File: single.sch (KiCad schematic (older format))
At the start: 8 parts, among them J1 Conn_01x01, J2 Conn_01x01, J3 Conn_01x01, J4 Conn_01x01, J5 Conn_01x01, J6 Conn_01x01

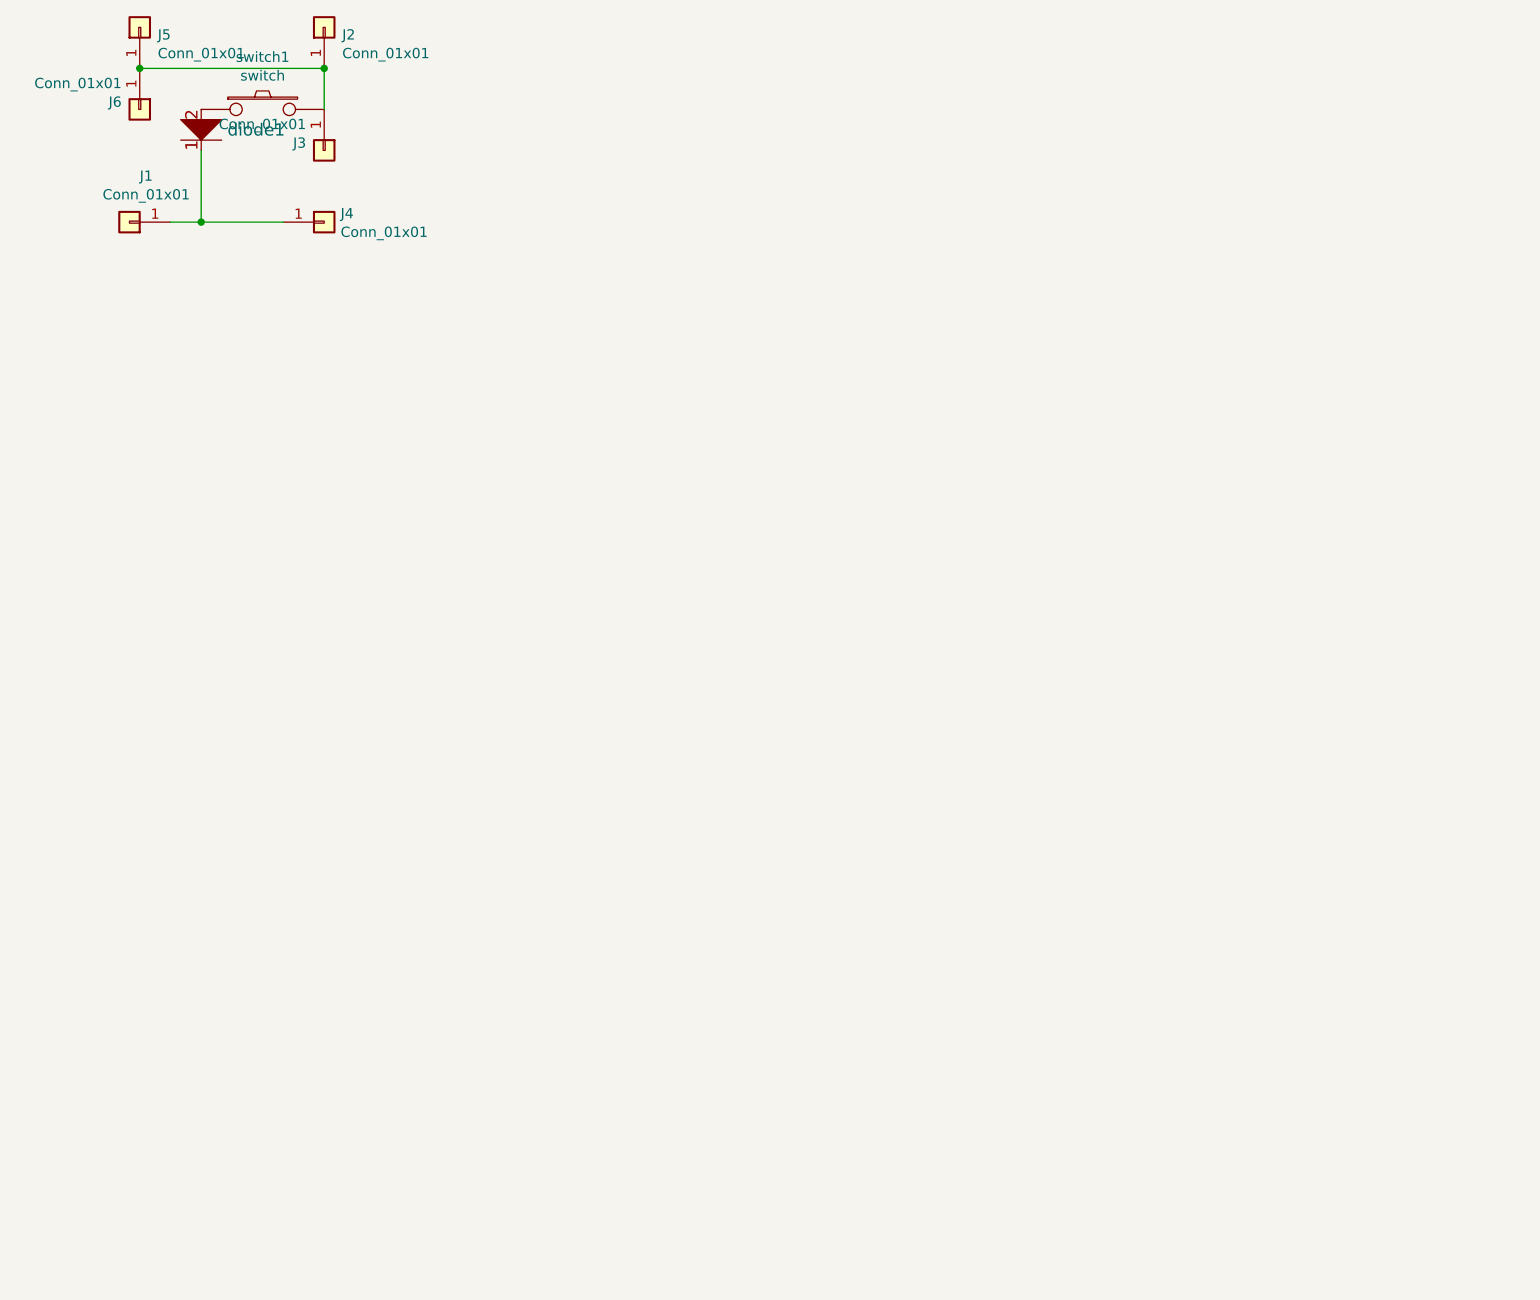
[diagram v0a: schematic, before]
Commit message: 6x5.
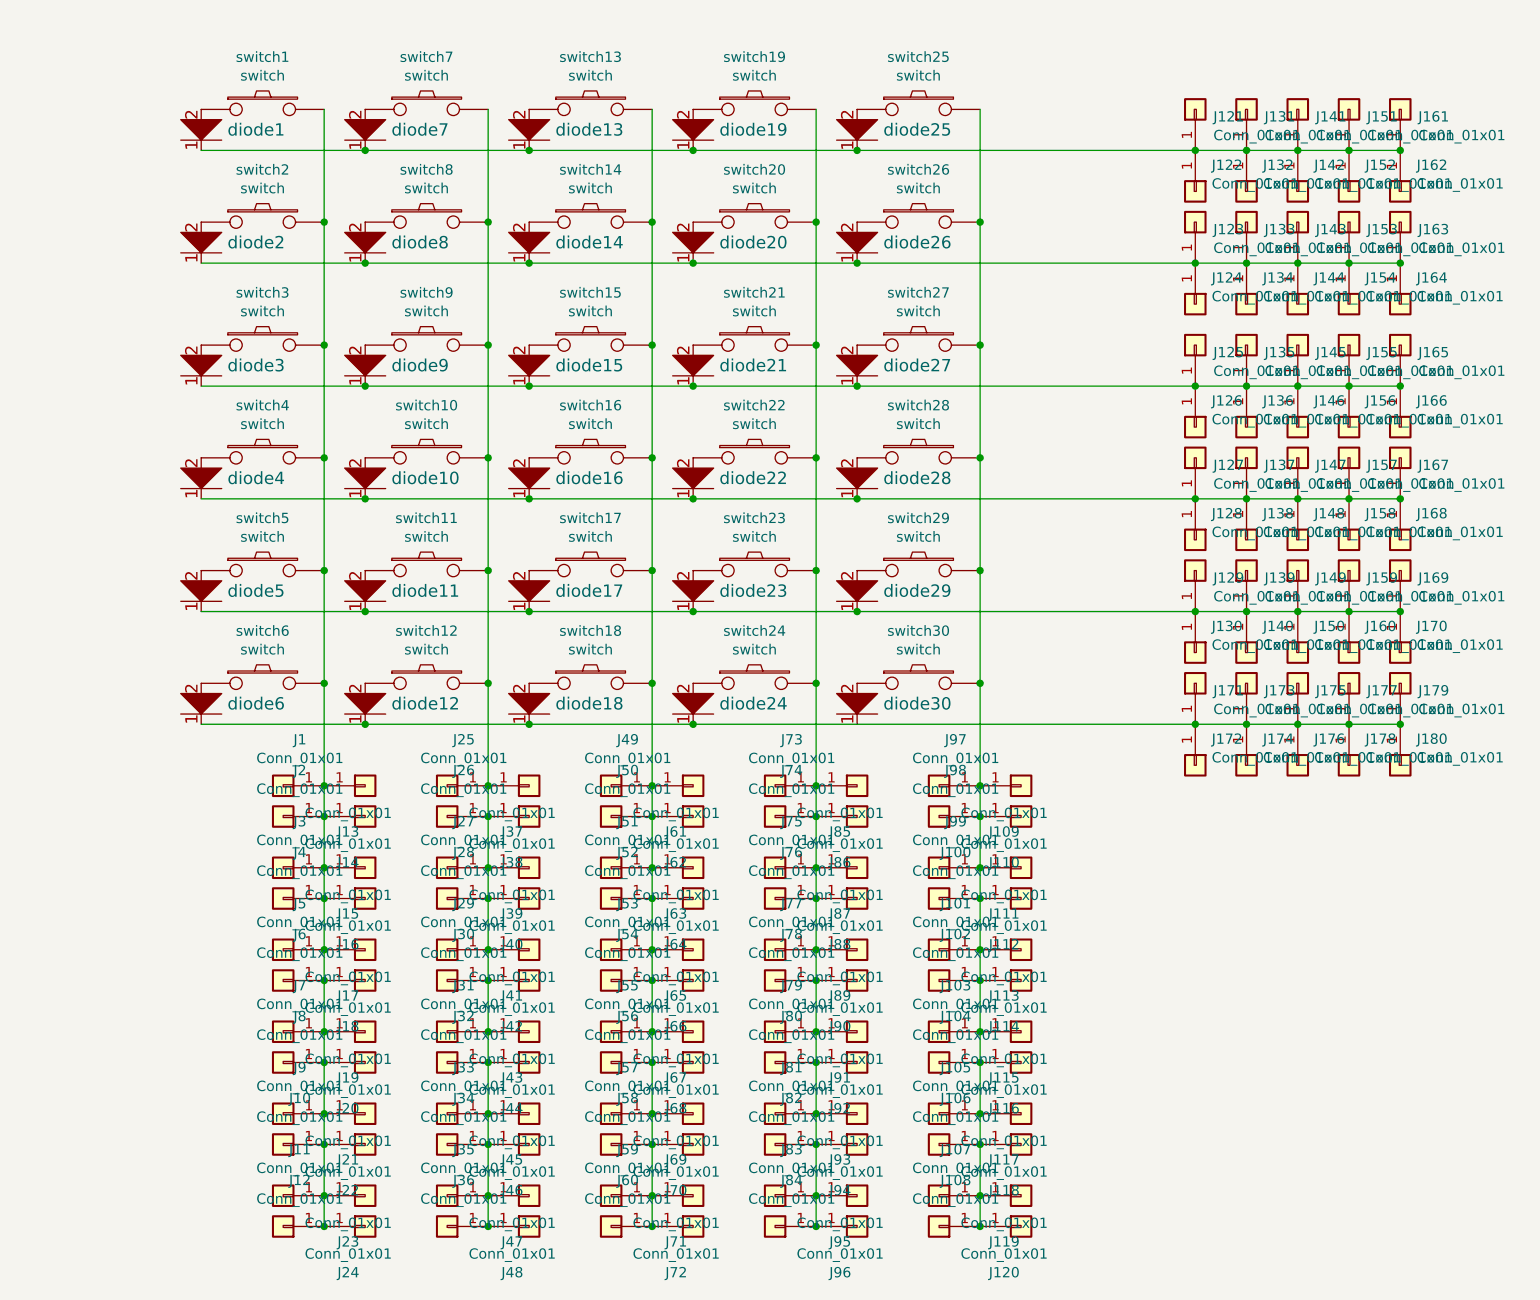
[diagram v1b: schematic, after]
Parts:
- added J10, J100, J101, J102, J103, J104, J105, J106, J107, J108, J109, J11, J110, J111, J112, J113, J114, J115, J116, J117, J118, J119, J12, J120, J121, J122, J123, J124, J125, J126, J127, J128, J129, J13, J130, J131, J132, J133, J134, J135, J136, J137, J138, J139, J14, J140, J141, J142, J143, J144, J145, J146, J147, J148, J149, J15, J150, J151, J152, J153, J154, J155, J156, J157, J158, J159, J16, J160, J161, J162, J163, J164, J165, J166, J167, J168, J169, J17, J170, J171, J172, J173, J174, J175, J176, J177, J178, J179, J18, J180, J19, J20, J21, J22, J23, J24, J25, J26, J27, J28, J29, J30, J31, J32, J33, J34, J35, J36, J37, J38, J39, J40, J41, J42, J43, J44, J45, J46, J47, J48, J49, J50, J51, J52, J53, J54, J55, J56, J57, J58, J59, J60, J61, J62, J63, J64, J65, J66, J67, J68, J69, J7, J70, J71, J72, J73, J74, J75, J76, J77, J78, J79, J8, J80, J81, J82, J83, J84, J85, J86, J87, J88, J89, J9, J90, J91, J92, J93, J94, J95, J96, J97, J98, J99: Conn_01x01, footprints:wirepad, symbol Connector_Generic:Conn_01x01
- added diode10, diode11, diode12, diode13, diode14, diode15, diode16, diode17, diode18, diode19, diode2, diode20, diode21, diode22, diode23, diode24, diode25, diode26, diode27, diode28, diode29, diode3, diode30, diode4, diode5, diode6, diode7, diode8, diode9: diode, footprints:diode, symbol single:diode
- added switch10, switch11, switch12, switch13, switch14, switch15, switch16, switch17, switch18, switch19, switch2, switch20, switch21, switch22, switch23, switch24, switch25, switch26, switch27, switch28, switch29, switch3, switch30, switch4, switch5, switch6, switch7, switch8, switch9: switch, footprints:1u-minimal, symbol single:switch
- switch1: footprint footprints:1u-flipped -> footprints:1u-minimal
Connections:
- net at J2.1 (Pin_1), J3.1 (Pin_1), J5.1 (Pin_1)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: now also J1.1 (Pin_1), J4.1 (Pin_1), J10.1 (Pin_1), J11.1 (Pin_1), J12.1 (Pin_1), J13.1 (Pin_1), J14.1 (Pin_1), J15.1 (Pin_1), J16.1 (Pin_1), J17.1 (Pin_1), J18.1 (Pin_1), J19.1 (Pin_1), J20.1 (Pin_1), J21.1 (Pin_1), J22.1 (Pin_1), J23.1 (Pin_1), J24.1 (Pin_1), J7.1 (Pin_1), J8.1 (Pin_1), J9.1 (Pin_1), switch2.2, switch3.2, switch4.2, switch5.2, switch6.2
- new net: J121.1 (Pin_1), J122.1 (Pin_1), J131.1 (Pin_1), J132.1 (Pin_1), J141.1 (Pin_1), J142.1 (Pin_1), J151.1 (Pin_1), J152.1 (Pin_1), J161.1 (Pin_1), J162.1 (Pin_1), diode1.1, diode13.1, diode19.1, diode25.1, diode7.1
- new net: J123.1 (Pin_1), J124.1 (Pin_1), J133.1 (Pin_1), J134.1 (Pin_1), J143.1 (Pin_1), J144.1 (Pin_1), J153.1 (Pin_1), J154.1 (Pin_1), J163.1 (Pin_1), J164.1 (Pin_1), diode14.1, diode2.1, diode20.1, diode26.1, diode8.1
- new net: diode2.2, switch2.1
- new net: J125.1 (Pin_1), J126.1 (Pin_1), J135.1 (Pin_1), J136.1 (Pin_1), J145.1 (Pin_1), J146.1 (Pin_1), J155.1 (Pin_1), J156.1 (Pin_1), J165.1 (Pin_1), J166.1 (Pin_1), diode15.1, diode21.1, diode27.1, diode3.1, diode9.1
- new net: diode3.2, switch3.1
- new net: J127.1 (Pin_1), J128.1 (Pin_1), J137.1 (Pin_1), J138.1 (Pin_1), J147.1 (Pin_1), J148.1 (Pin_1), J157.1 (Pin_1), J158.1 (Pin_1), J167.1 (Pin_1), J168.1 (Pin_1), diode10.1, diode16.1, diode22.1, diode28.1, diode4.1
- new net: diode4.2, switch4.1
- new net: J129.1 (Pin_1), J130.1 (Pin_1), J139.1 (Pin_1), J140.1 (Pin_1), J149.1 (Pin_1), J150.1 (Pin_1), J159.1 (Pin_1), J160.1 (Pin_1), J169.1 (Pin_1), J170.1 (Pin_1), diode11.1, diode17.1, diode23.1, diode29.1, diode5.1
- new net: diode5.2, switch5.1
- new net: J171.1 (Pin_1), J172.1 (Pin_1), J173.1 (Pin_1), J174.1 (Pin_1), J175.1 (Pin_1), J176.1 (Pin_1), J177.1 (Pin_1), J178.1 (Pin_1), J179.1 (Pin_1), J180.1 (Pin_1), diode12.1, diode18.1, diode24.1, diode30.1, diode6.1
- new net: diode6.2, switch6.1
- new net: diode7.2, switch7.1
- new net: J25.1 (Pin_1), J26.1 (Pin_1), J27.1 (Pin_1), J28.1 (Pin_1), J29.1 (Pin_1), J30.1 (Pin_1), J31.1 (Pin_1), J32.1 (Pin_1), J33.1 (Pin_1), J34.1 (Pin_1), J35.1 (Pin_1), J36.1 (Pin_1), J37.1 (Pin_1), J38.1 (Pin_1), J39.1 (Pin_1), J40.1 (Pin_1), J41.1 (Pin_1), J42.1 (Pin_1), J43.1 (Pin_1), J44.1 (Pin_1), J45.1 (Pin_1), J46.1 (Pin_1), J47.1 (Pin_1), J48.1 (Pin_1), switch10.2, switch11.2, switch12.2, switch7.2, switch8.2, switch9.2
- new net: diode8.2, switch8.1
- new net: diode9.2, switch9.1
- new net: diode10.2, switch10.1
- new net: diode11.2, switch11.1
- new net: diode12.2, switch12.1
- new net: diode13.2, switch13.1
- new net: J49.1 (Pin_1), J50.1 (Pin_1), J51.1 (Pin_1), J52.1 (Pin_1), J53.1 (Pin_1), J54.1 (Pin_1), J55.1 (Pin_1), J56.1 (Pin_1), J57.1 (Pin_1), J58.1 (Pin_1), J59.1 (Pin_1), J60.1 (Pin_1), J61.1 (Pin_1), J62.1 (Pin_1), J63.1 (Pin_1), J64.1 (Pin_1), J65.1 (Pin_1), J66.1 (Pin_1), J67.1 (Pin_1), J68.1 (Pin_1), J69.1 (Pin_1), J70.1 (Pin_1), J71.1 (Pin_1), J72.1 (Pin_1), switch13.2, switch14.2, switch15.2, switch16.2, switch17.2, switch18.2
- new net: diode14.2, switch14.1
- new net: diode15.2, switch15.1
- new net: diode16.2, switch16.1
- new net: diode17.2, switch17.1
- new net: diode18.2, switch18.1
- new net: diode19.2, switch19.1
- new net: J73.1 (Pin_1), J74.1 (Pin_1), J75.1 (Pin_1), J76.1 (Pin_1), J77.1 (Pin_1), J78.1 (Pin_1), J79.1 (Pin_1), J80.1 (Pin_1), J81.1 (Pin_1), J82.1 (Pin_1), J83.1 (Pin_1), J84.1 (Pin_1), J85.1 (Pin_1), J86.1 (Pin_1), J87.1 (Pin_1), J88.1 (Pin_1), J89.1 (Pin_1), J90.1 (Pin_1), J91.1 (Pin_1), J92.1 (Pin_1), J93.1 (Pin_1), J94.1 (Pin_1), J95.1 (Pin_1), J96.1 (Pin_1), switch19.2, switch20.2, switch21.2, switch22.2, switch23.2, switch24.2
- new net: diode20.2, switch20.1
- new net: diode21.2, switch21.1
- new net: diode22.2, switch22.1
- new net: diode23.2, switch23.1
- new net: diode24.2, switch24.1
- new net: diode25.2, switch25.1
- new net: J100.1 (Pin_1), J101.1 (Pin_1), J102.1 (Pin_1), J103.1 (Pin_1), J104.1 (Pin_1), J105.1 (Pin_1), J106.1 (Pin_1), J107.1 (Pin_1), J108.1 (Pin_1), J109.1 (Pin_1), J110.1 (Pin_1), J111.1 (Pin_1), J112.1 (Pin_1), J113.1 (Pin_1), J114.1 (Pin_1), J115.1 (Pin_1), J116.1 (Pin_1), J117.1 (Pin_1), J118.1 (Pin_1), J119.1 (Pin_1), J120.1 (Pin_1), J97.1 (Pin_1), J98.1 (Pin_1), J99.1 (Pin_1), switch25.2, switch26.2, switch27.2, switch28.2, switch29.2, switch30.2
- new net: diode26.2, switch26.1
- new net: diode27.2, switch27.1
- new net: diode28.2, switch28.1
- new net: diode29.2, switch29.1
- new net: diode30.2, switch30.1
